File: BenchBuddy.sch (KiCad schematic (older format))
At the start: 0 parts

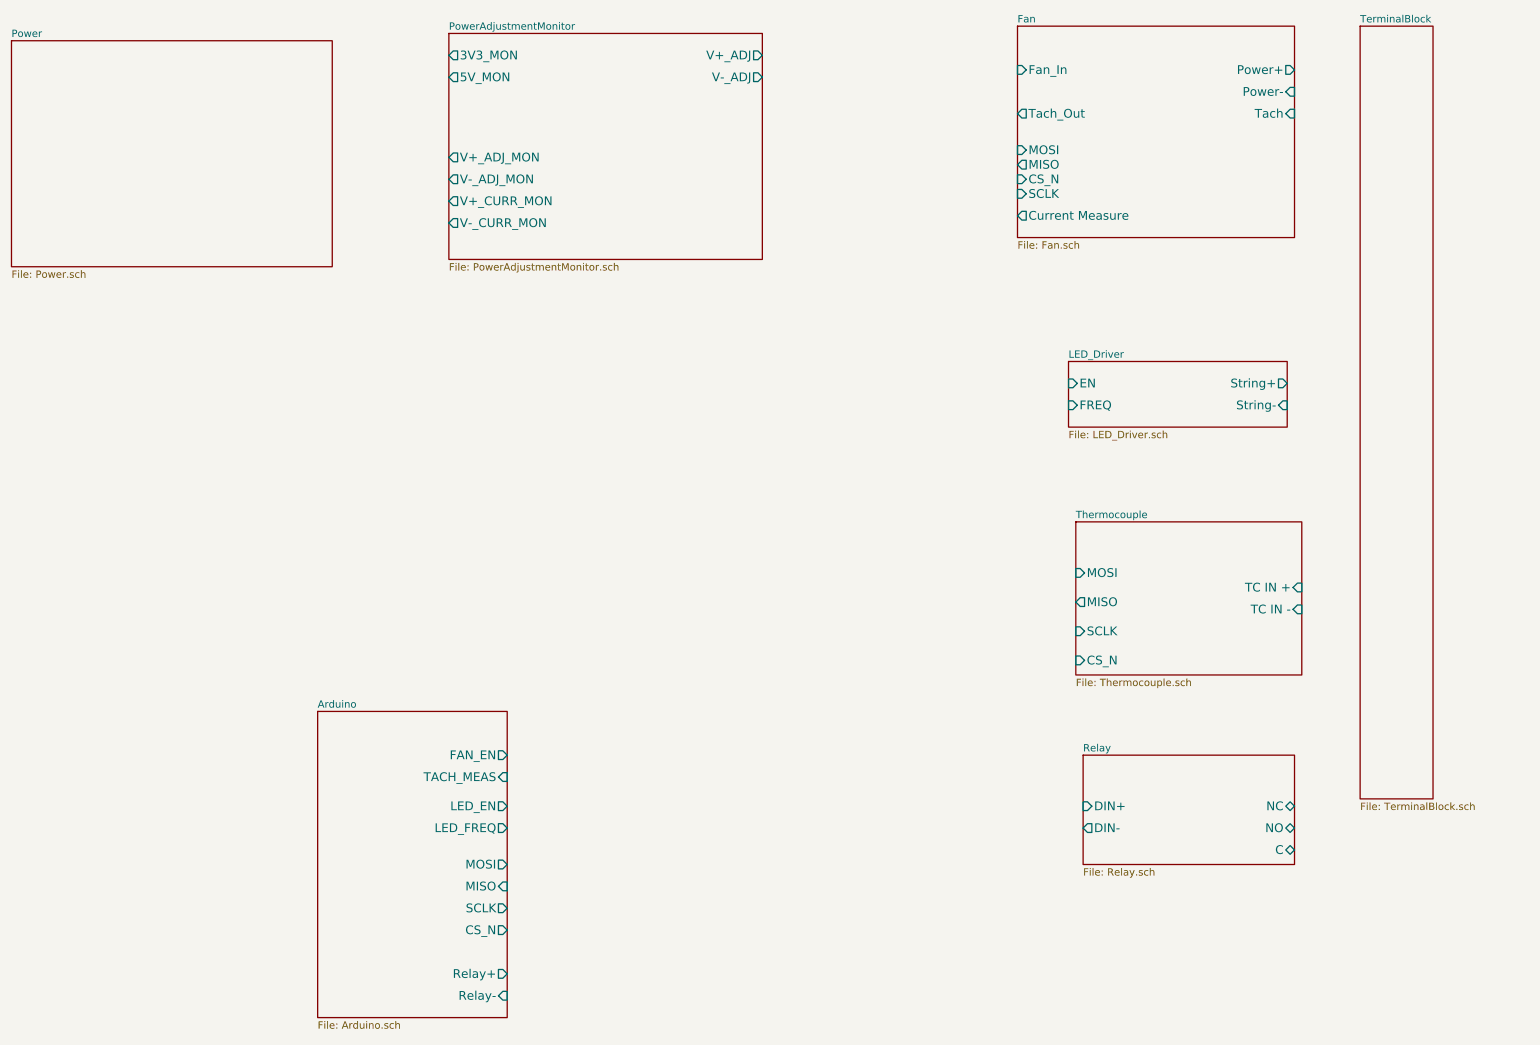
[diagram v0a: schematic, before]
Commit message: Overall Schematic
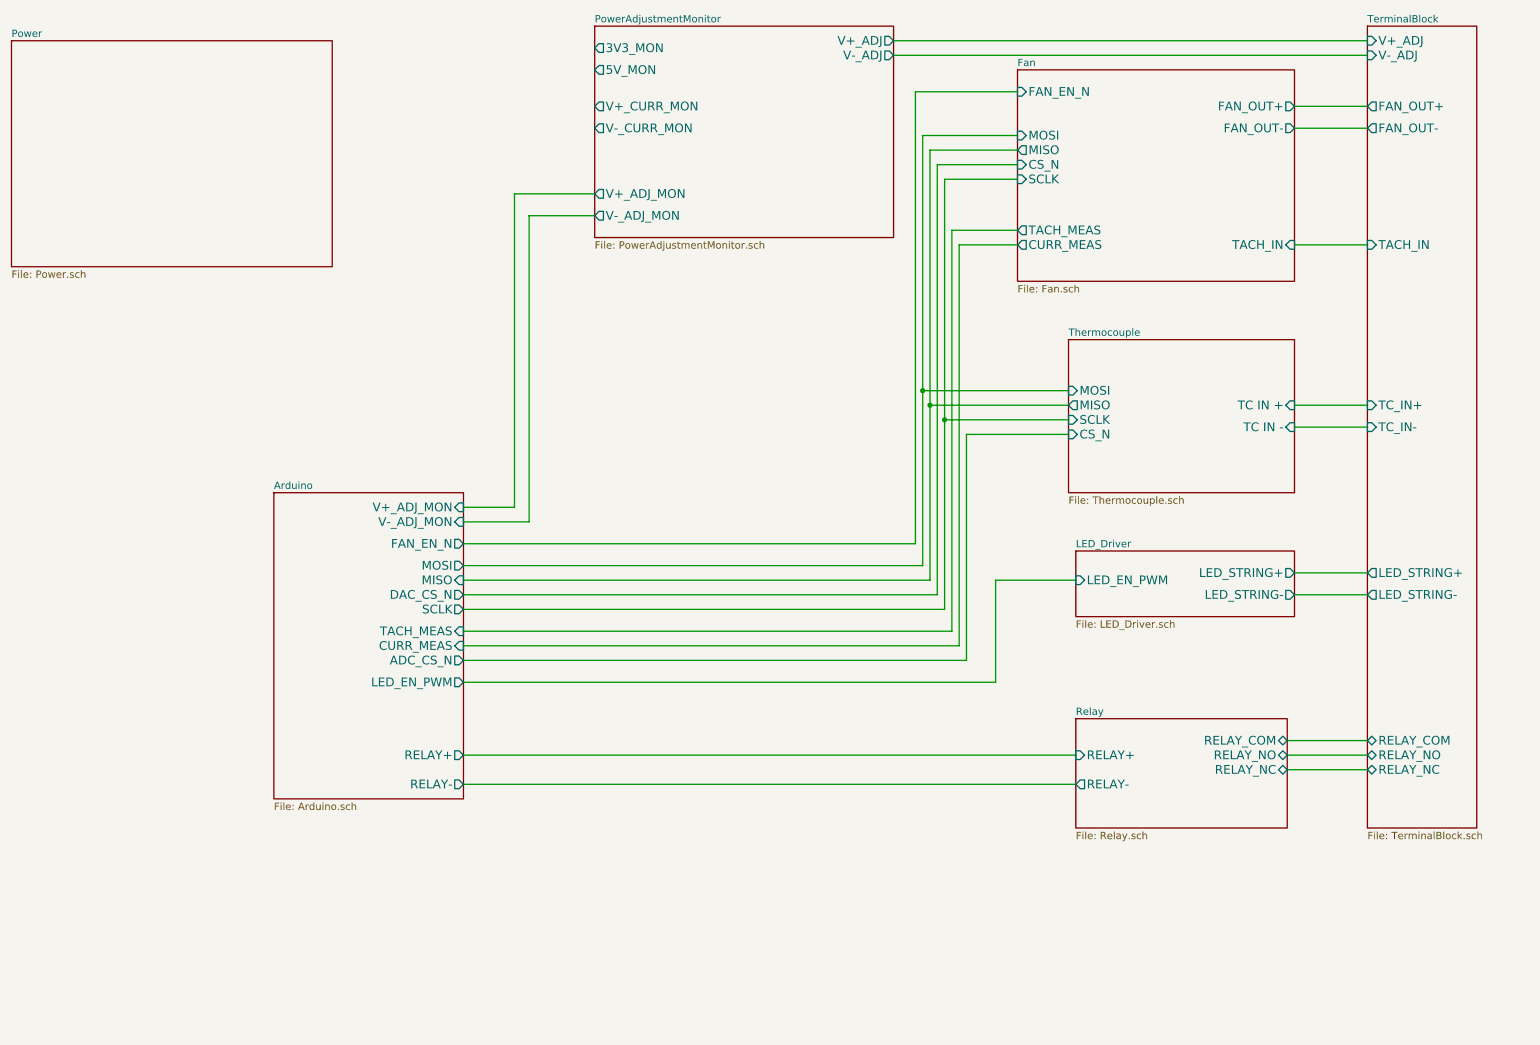
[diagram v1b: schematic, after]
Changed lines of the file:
@@
 Sheet 1 9
 Title ""
-Date "22 sep 2013"
+Date "28 sep 2013"
 Rev ""
 Comp ""
@@
 $EndDescr
 $Sheet
-S 3050 5500 1300 2100
-U 5237E014
-F0 "Arduino" 50
-F1 "Arduino.sch" 50
-F2 "FAN_EN" O R 4350 5800 60
-F3 "TACH_MEAS" I R 4350 5950 60
-F4 "LED_EN" O R 4350 6150 60
-F5 "LED_FREQ" O R 4350 6300 60
-F6 "MOSI" O R 4350 6550 60
-F7 "MISO" I R 4350 6700 60
-F8 "SCLK" O R 4350 6850 60
-F9 "CS_N" O R 4350 7000 60
-F10 "Relay+" O R 4350 7300 60
-F11 "Relay-" I R 4350 7450 60
-$EndSheet
-$Sheet
-S 8250 4200 1550 1050
+S 8200 2950 1550 1050
 U 5237E11D
 F0 "Thermocouple" 50
 F1 "Thermocouple.sch" 50
-F2 "TC IN +" I R 9800 4650 60
-F3 "TC IN -" I R 9800 4800 60
-F4 "MOSI" I L 8250 4550 60
-F5 "MISO" O L 8250 4750 60
-F6 "SCLK" I L 8250 4950 60
-F7 "CS_N" I L 8250 5150 60
+F2 "TC IN +" I R 9750 3400 60
+F3 "TC IN -" I R 9750 3550 60
+F4 "MOSI" I L 8200 3300 60
+F5 "MISO" O L 8200 3400 60
+F6 "SCLK" I L 8200 3500 60
+F7 "CS_N" I L 8200 3600 60
 $EndSheet
 $Sheet
@@
 $EndSheet
 $Sheet
-S 8200 3100 1500 450
+S 8250 4400 1500 450
 U 5237E1C9
 F0 "LED_Driver" 50
 F1 "LED_Driver.sch" 50
-F2 "EN" I L 8200 3250 60
-F3 "FREQ" I L 8200 3400 60
-F4 "String+" O R 9700 3250 60
-F5 "String-" I R 9700 3400 60
-$EndSheet
-$Sheet
-S 7850 800  1900 1450
+F2 "LED_EN_PWM" I L 8250 4600 60
+F3 "LED_STRING+" O R 9750 4550 60
+F4 "LED_STRING-" O R 9750 4700 60
+$EndSheet
+$Sheet
+S 7850 1100 1900 1450
 U 5237E1FA
 F0 "Fan" 50
 F1 "Fan.sch" 50
-F2 "Fan_In" I L 7850 1100 60
-F3 "Tach_Out" O L 7850 1400 60
-F4 "Power+" O R 9750 1100 60
-F5 "Power-" I R 9750 1250 60
-F6 "Tach" I R 9750 1400 60
-F7 "MOSI" I L 7850 1650 60
-F8 "MISO" O L 7850 1750 60
-F9 "CS_N" I L 7850 1850 60
-F10 "SCLK" I L 7850 1950 60
-F11 "Current Measure" O L 7850 2100 60
-$EndSheet
-$Sheet
-S 10200 800  500  5300
+F2 "MOSI" I L 7850 1550 60
+F3 "MISO" O L 7850 1650 60
+F4 "CS_N" I L 7850 1750 60
+F5 "SCLK" I L 7850 1850 60
+F6 "FAN_EN_N" I L 7850 1250 60
+F7 "TACH_MEAS" O L 7850 2200 60
+F8 "FAN_OUT+" O R 9750 1350 60
+F9 "FAN_OUT-" O R 9750 1500 60
+F10 "TACH_IN" I R 9750 2300 60
+F11 "CURR_MEAS" O L 7850 2300 60
+$EndSheet
+$Sheet
+S 8250 5550 1450 750
+U 5237E13C
+F0 "Relay" 50
+F1 "Relay.sch" 50
+F2 "RELAY+" I L 8250 5800 60
+F3 "RELAY-" O L 8250 6000 60
+F4 "RELAY_NC" B R 9700 5900 60
+F5 "RELAY_NO" B R 9700 5800 60
+F6 "RELAY_COM" B R 9700 5700 60
+$EndSheet
+$Sheet
+S 4950 800  2050 1450
+U 523E68DB
+F0 "PowerAdjustmentMonitor" 50
+F1 "PowerAdjustmentMonitor.sch" 50
+F2 "V+_ADJ" O R 7000 900 60
+F3 "V-_ADJ" O R 7000 1000 60
+F4 "3V3_MON" O L 4950 950 60
+F5 "5V_MON" O L 4950 1100 60
+F6 "V+_ADJ_MON" O L 4950 1950 60
+F7 "V-_ADJ_MON" O L 4950 2100 60
+F8 "V+_CURR_MON" O L 4950 1350 60
+F9 "V-_CURR_MON" O L 4950 1500 60
+$EndSheet
+Wire Wire Line
+	4050 4100 4400 4100
+Wire Wire Line
+	4400 4100 4400 1950
+Wire Wire Line
+	4400 1950 4950 1950
+Wire Wire Line
+	4950 2100 4500 2100
+Wire Wire Line
+	4500 2100 4500 4200
+Wire Wire Line
+	4500 4200 4050 4200
+Wire Wire Line
+	4050 4350 7150 4350
+Wire Wire Line
+	7150 4350 7150 1250
+Wire Wire Line
+	7150 1250 7850 1250
+Wire Wire Line
+	7850 1550 7200 1550
+Wire Wire Line
+	7200 1550 7200 4500
+Wire Wire Line
+	7200 4500 4050 4500
+Wire Wire Line
+	4050 4600 7250 4600
+Wire Wire Line
+	7250 4600 7250 1650
+Wire Wire Line
+	7250 1650 7850 1650
+Wire Wire Line
+	7850 1750 7300 1750
+Wire Wire Line
+	7300 1750 7300 4700
+Wire Wire Line
+	7300 4700 4050 4700
+Wire Wire Line
+	4050 4800 7350 4800
+Wire Wire Line
+	7350 4800 7350 1850
+Wire Wire Line
+	7350 1850 7850 1850
+Wire Wire Line
+	7850 2200 7400 2200
+Wire Wire Line
+	7400 2200 7400 4950
+Wire Wire Line
+	7400 4950 4050 4950
+Wire Wire Line
+	4050 5050 7450 5050
+Wire Wire Line
+	7450 5050 7450 2300
+Wire Wire Line
+	7450 2300 7850 2300
+Wire Wire Line
+	8200 3300 7200 3300
+Connection ~ 7200 3300
+Wire Wire Line
+	8200 3400 7250 3400
+Connection ~ 7250 3400
+$Sheet
+S 2750 4000 1300 2100
+U 5237E014
+F0 "Arduino" 50
+F1 "Arduino.sch" 50
+F2 "TACH_MEAS" I R 4050 4950 60
+F3 "MOSI" O R 4050 4500 60
+F4 "MISO" I R 4050 4600 60
+F5 "SCLK" O R 4050 4800 60
+F6 "FAN_EN_N" O R 4050 4350 60
+F7 "CURR_MEAS" I R 4050 5050 60
+F8 "RELAY+" O R 4050 5800 60
+F9 "RELAY-" O R 4050 6000 60
+F10 "V+_ADJ_MON" I R 4050 4100 60
+F11 "V-_ADJ_MON" I R 4050 4200 60
+F12 "LED_EN_PWM" O R 4050 5300 60
+F13 "DAC_CS_N" O R 4050 4700 60
+F14 "ADC_CS_N" O R 4050 5150 60
+$EndSheet
+Wire Wire Line
+	7350 3500 8200 3500
+Connection ~ 7350 3500
+Wire Wire Line
+	8200 3600 7500 3600
+Wire Wire Line
+	7500 3600 7500 5150
+Wire Wire Line
+	7500 5150 4050 5150
+Wire Wire Line
+	4050 5300 7700 5300
+Wire Wire Line
+	7700 5300 7700 4600
+Wire Wire Line
+	7700 4600 8250 4600
+Wire Wire Line
+	4050 5800 8250 5800
+Wire Wire Line
+	8250 6000 4050 6000
+$Sheet
+S 10250 800  750  5500
 U 5237E269
 F0 "TerminalBlock" 50
 F1 "TerminalBlock.sch" 50
-$EndSheet
-$Sheet
-S 8300 5800 1450 750
-U 5237E13C
-F0 "Relay" 50
-F1 "Relay.sch" 50
-F2 "DIN+" I L 8300 6150 60
-F3 "DIN-" O L 8300 6300 60
-F4 "NC" B R 9750 6150 60
-F5 "NO" B R 9750 6300 60
-F6 "C" B R 9750 6450 60
-$EndSheet
-$Sheet
-S 3950 850  2150 1550
-U 523E68DB
-F0 "PowerAdjustmentMonitor" 50
-F1 "PowerAdjustmentMonitor.sch" 50
-F2 "V+_ADJ" O R 6100 1000 60
-F3 "V-_ADJ" O R 6100 1150 60
-F4 "3V3_MON" O L 3950 1000 60
-F5 "5V_MON" O L 3950 1150 60
-F6 "V+_ADJ_MON" O L 3950 1700 60
-F7 "V-_ADJ_MON" O L 3950 1850 60
-F8 "V+_CURR_MON" O L 3950 2000 60
-F9 "V-_CURR_MON" O L 3950 2150 60
-$EndSheet
+F2 "V+_ADJ" I L 10250 900 60
+F3 "V-_ADJ" I L 10250 1000 60
+F4 "FAN_OUT+" O L 10250 1350 60
+F5 "FAN_OUT-" O L 10250 1500 60
+F6 "TACH_IN" I L 10250 2300 60
+F7 "TC_IN+" I L 10250 3400 60
+F8 "TC_IN-" I L 10250 3550 60
+F9 "LED_STRING+" O L 10250 4550 60
+F10 "LED_STRING-" O L 10250 4700 60
+F11 "RELAY_COM" B L 10250 5700 60
+F12 "RELAY_NO" B L 10250 5800 60
+F13 "RELAY_NC" B L 10250 5900 60
+$EndSheet
+Wire Wire Line
+	7000 900  10250 900
+Wire Wire Line
+	7000 1000 10250 1000
+Wire Wire Line
+	9750 1350 10250 1350
+Wire Wire Line
+	9750 1500 10250 1500
+Wire Wire Line
+	9750 2300 10250 2300
+Wire Wire Line
+	9750 3400 10250 3400
+Wire Wire Line
+	9750 3550 10250 3550
+Wire Wire Line
+	9750 4550 10250 4550
+Wire Wire Line
+	9750 4700 10250 4700
+Wire Wire Line
+	9700 5700 10250 5700
+Wire Wire Line
+	9700 5800 10250 5800
+Wire Wire Line
+	9700 5900 10250 5900
 $EndSCHEMATC
